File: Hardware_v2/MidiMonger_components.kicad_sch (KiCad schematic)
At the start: 66 parts, among them J1 Conn_01x09_Male, J2 Conn_01x09_Male, J3 Conn_01x08_Male, J4 Conn_01x08_Male, J5 SWD_Header, J6 Eurorack_10_pin_power, J7 UART_Test, U1 STM32F446RETx, U2 TL074, U3 74HCT244, U4 MAX5134, U5 6N137, U6 LM1117-3.3, U7 LM1117-5.0, Y1 8MHz 20pF

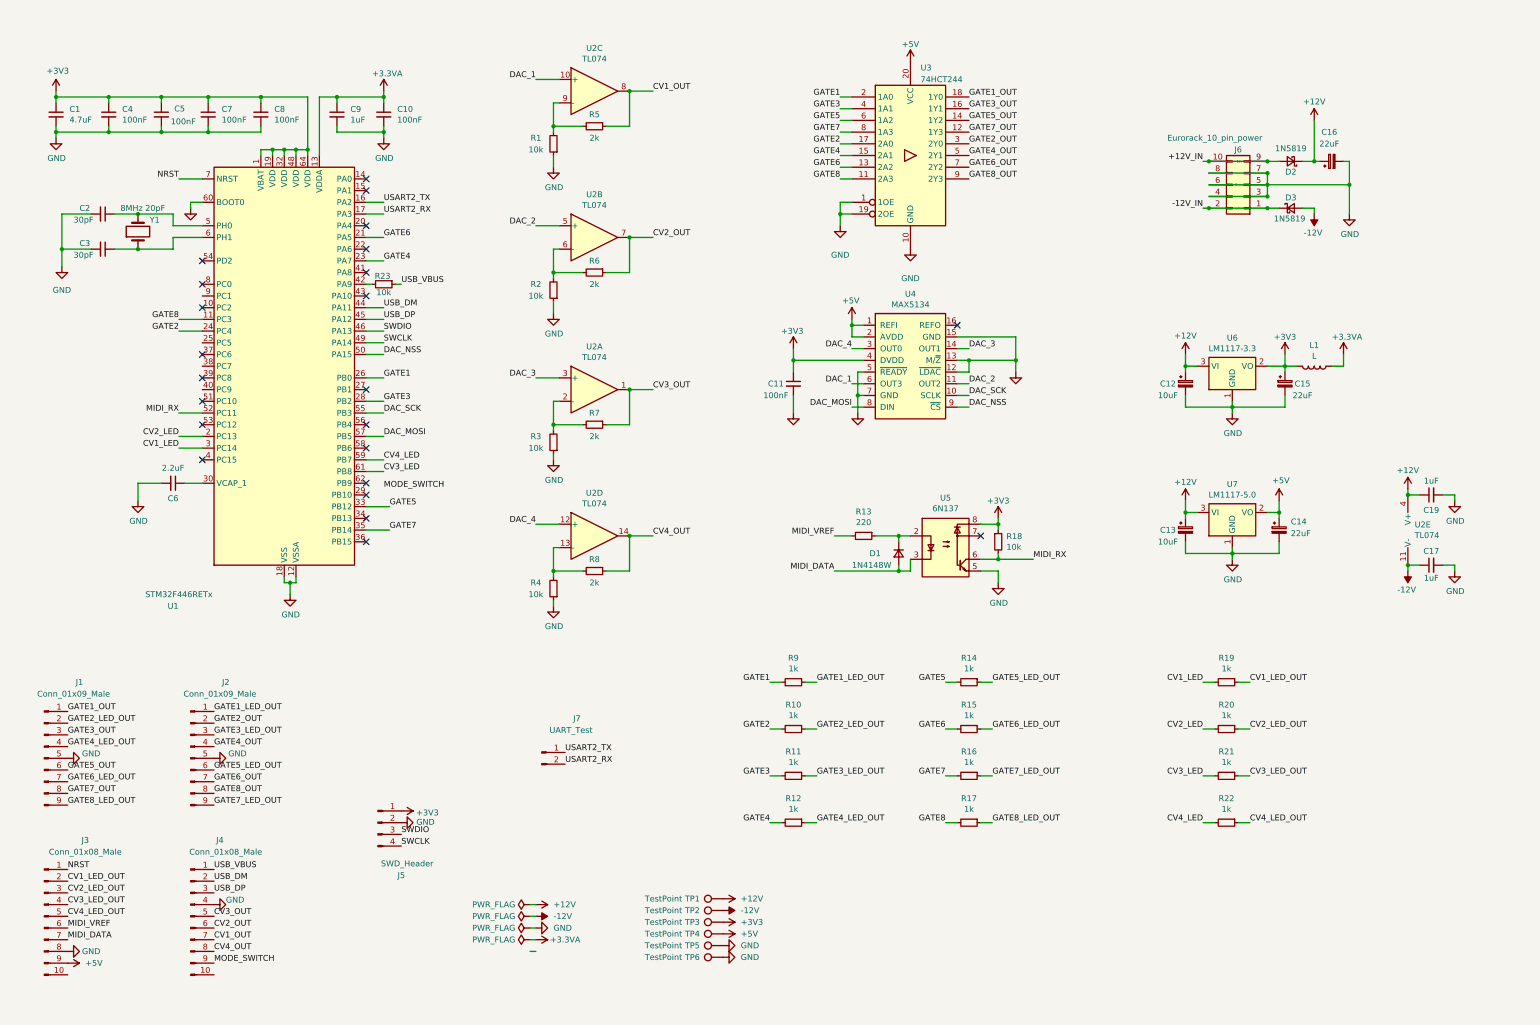
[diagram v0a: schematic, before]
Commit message: Hardware layout
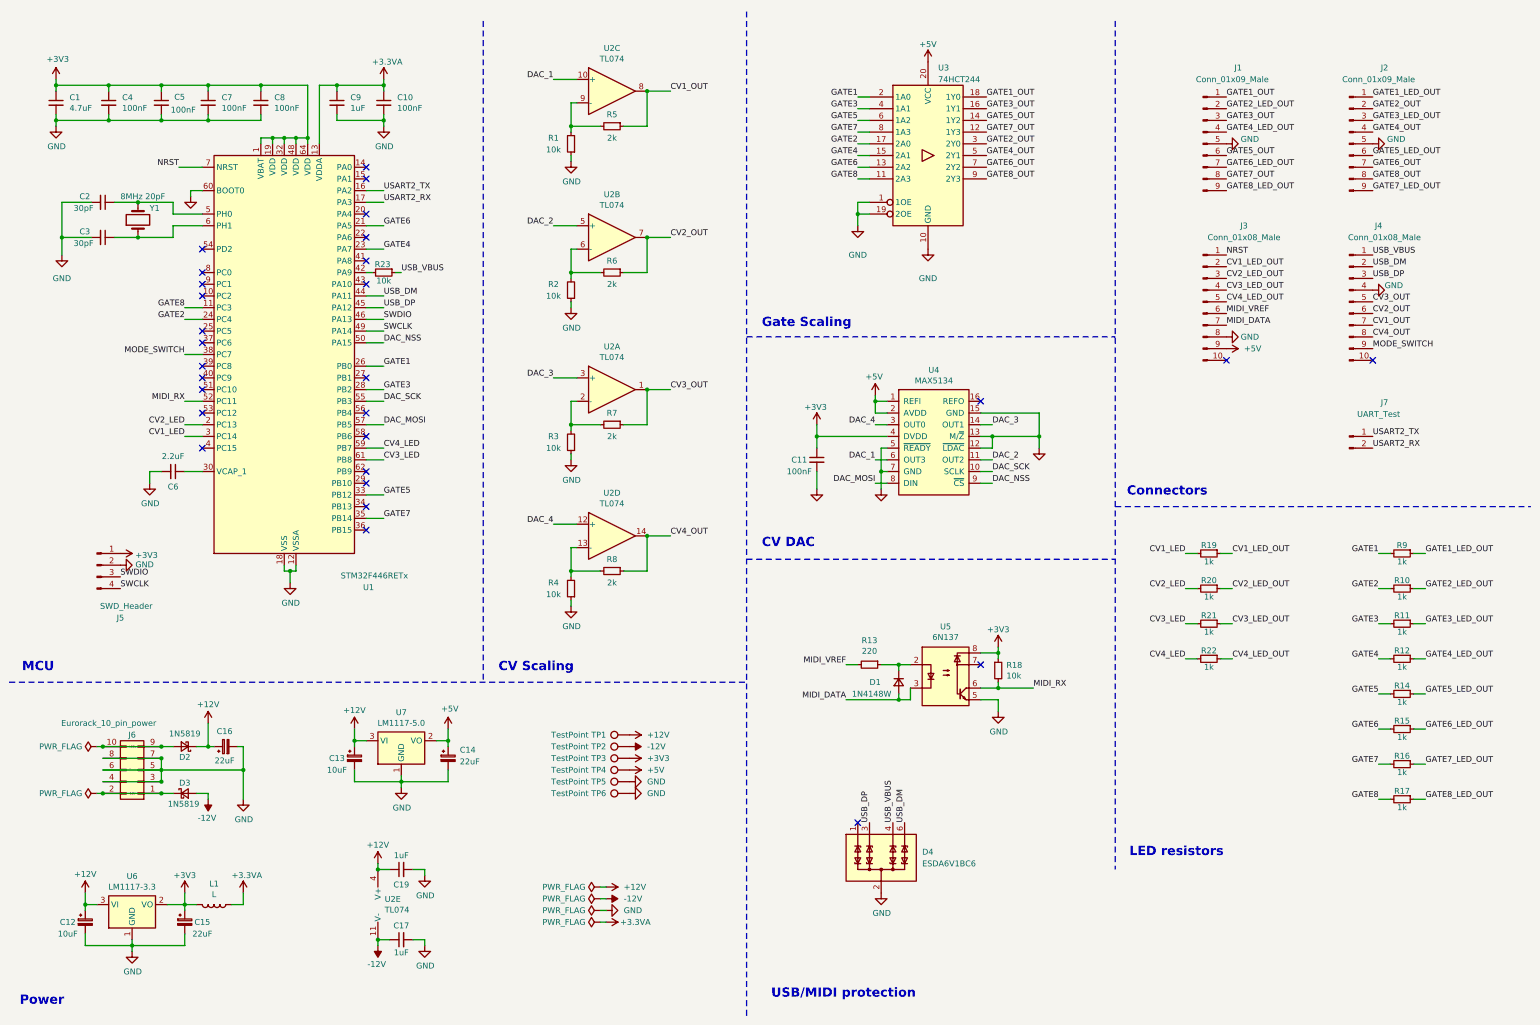
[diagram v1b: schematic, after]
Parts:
- added D4: ESDA6V1BC6, Package_TO_SOT_SMD:SOT-23-6, symbol Power_Protection:ESDA6V1BC6
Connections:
- net GND: now also D4.2 (COM), D4.5 (COM)
- net MODE_SWITCH: now also U1.38 (PC7)
- net USB_DM: now also D4.6 (TVS4)
- net USB_DP: now also D4.3 (TVS2)
- net USB_VBUS: now also D4.4 (TVS3)
- net +12V_IN: no longer names the net of D2.2 (A), J6.10 (Pin_10), J6.9 (Pin_9)
- net -12V_IN: no longer names the net of D3.1 (K), J6.1 (Pin_1), J6.2 (Pin_2)
- no-connect marks 23 -> 29
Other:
- note added: "CV DAC"
- note added: "CV Scaling"
- note added: "Connectors"
- note added: "Gate Scaling"
- note added: "LED resistors"
- note added: "MCU"
- note added: "Power"
- note added: "USB/MIDI protection"
- moved on the sheet: C1, C10, C11, C12, C13, C14, C15, C16, C17, C19, C2, C3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
